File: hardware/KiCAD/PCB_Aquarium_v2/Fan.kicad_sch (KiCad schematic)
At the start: 8 parts, among them J2 Conn_01x02, J3 Conn_01x02, J4 Conn_01x02, J5 Conn_01x02

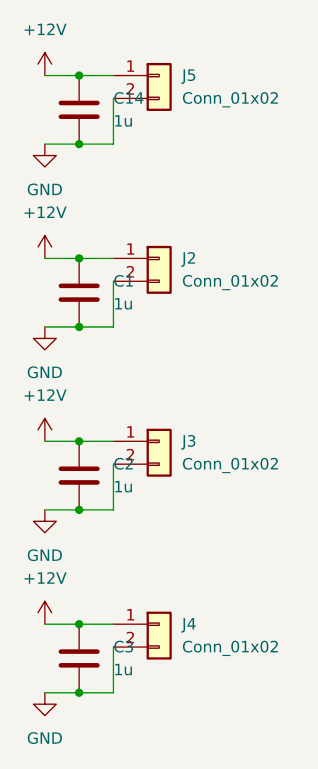
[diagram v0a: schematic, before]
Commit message: PCB principal finis
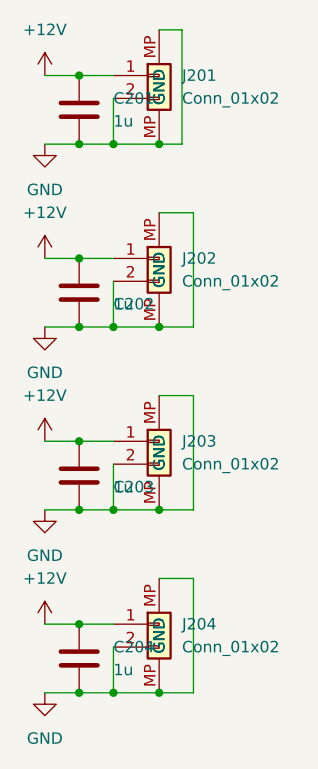
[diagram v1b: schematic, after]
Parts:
- J201: renamed from J5; footprint Connector_JST:JST_EH_B2B-EH-A_1x02_P2.50mm_Vertical -> Connector_JST:JST_SH_BM02B-SRSS-TB_1x02-1MP_P1.00mm_Vertical; symbol Connector_Generic:Conn_01x02 -> my_lib:JST_SH_2_Vertical
- J202: renamed from J2; footprint Connector_JST:JST_EH_B2B-EH-A_1x02_P2.50mm_Vertical -> Connector_JST:JST_SH_BM02B-SRSS-TB_1x02-1MP_P1.00mm_Vertical; symbol Connector_Generic:Conn_01x02 -> my_lib:JST_SH_2_Vertical
- J203: renamed from J3; footprint Connector_JST:JST_EH_B2B-EH-A_1x02_P2.50mm_Vertical -> Connector_JST:JST_SH_BM02B-SRSS-TB_1x02-1MP_P1.00mm_Vertical; symbol Connector_Generic:Conn_01x02 -> my_lib:JST_SH_2_Vertical
- J204: renamed from J4; footprint Connector_JST:JST_EH_B2B-EH-A_1x02_P2.50mm_Vertical -> Connector_JST:JST_SH_BM02B-SRSS-TB_1x02-1MP_P1.00mm_Vertical; symbol Connector_Generic:Conn_01x02 -> my_lib:JST_SH_2_Vertical
- renumbered C14 to C201, C1 to C202, C2 to C203, C3 to C204
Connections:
- net GND: now also J201.MP (GND), J202.MP (GND), J203.MP (GND), J204.MP (GND)
